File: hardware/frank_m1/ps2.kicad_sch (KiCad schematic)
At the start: 14 parts, among them J4 MDC-036

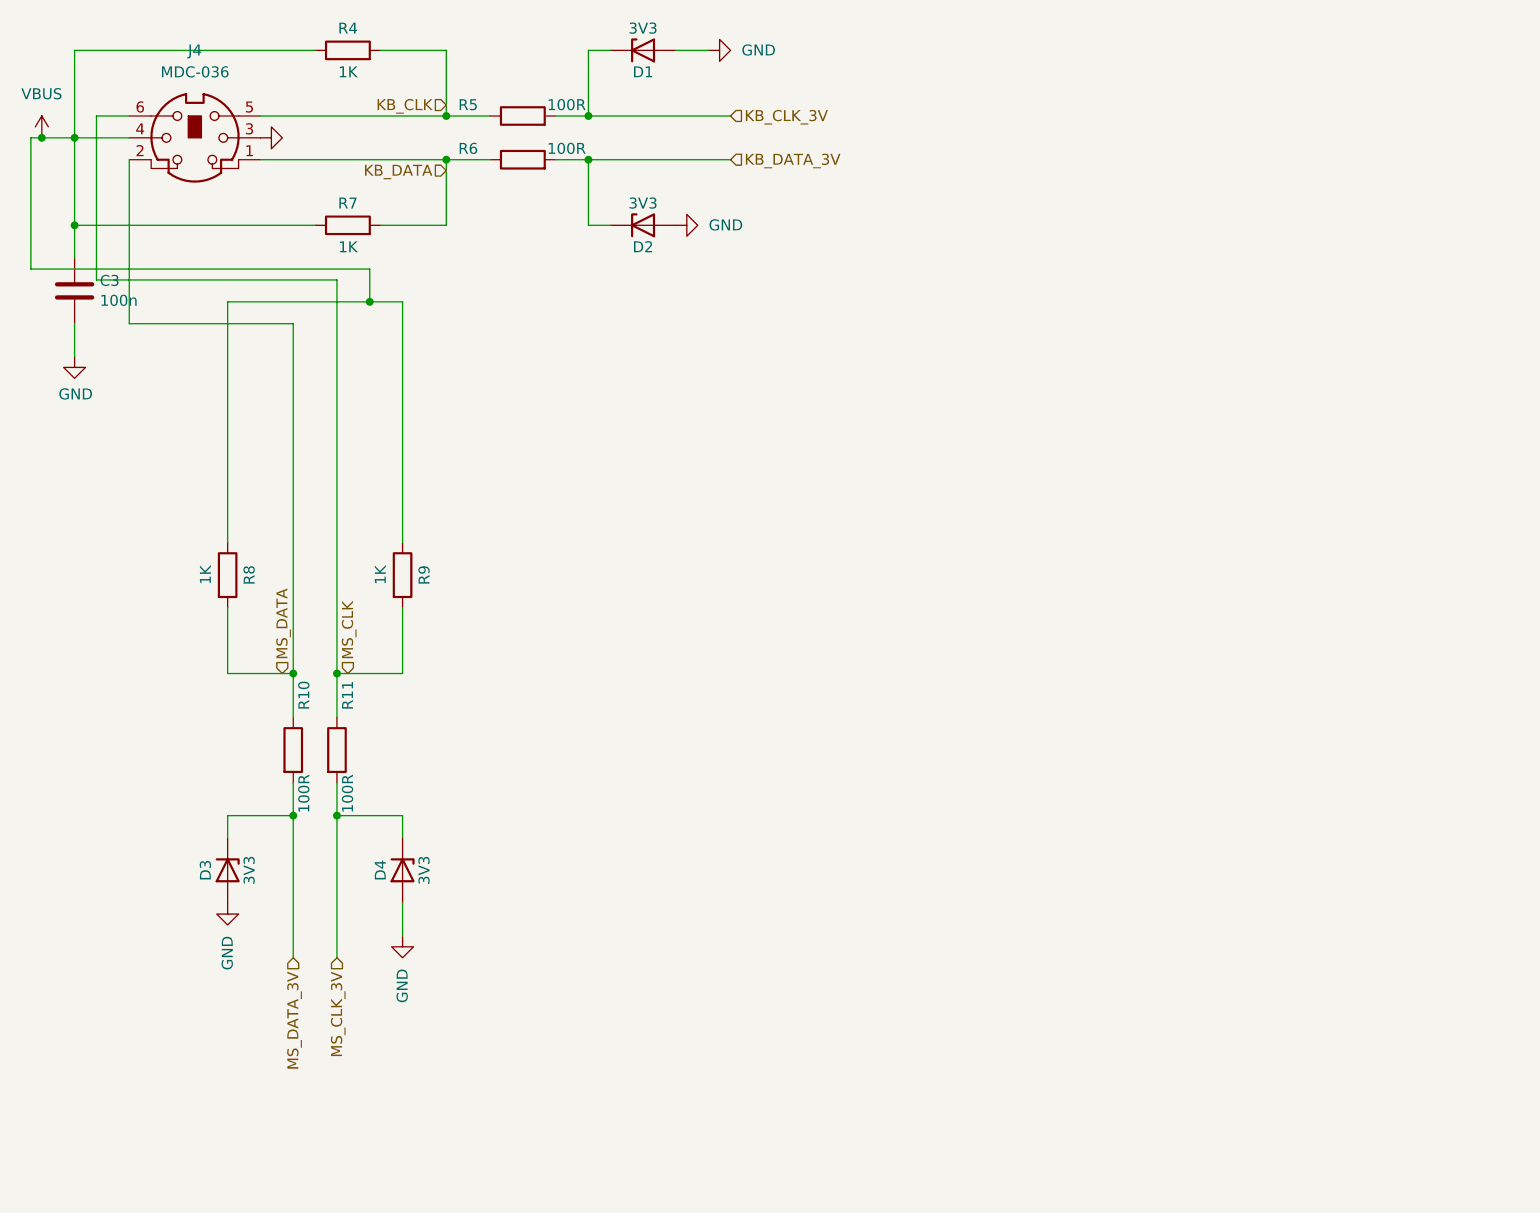
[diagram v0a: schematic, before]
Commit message: Minor updates
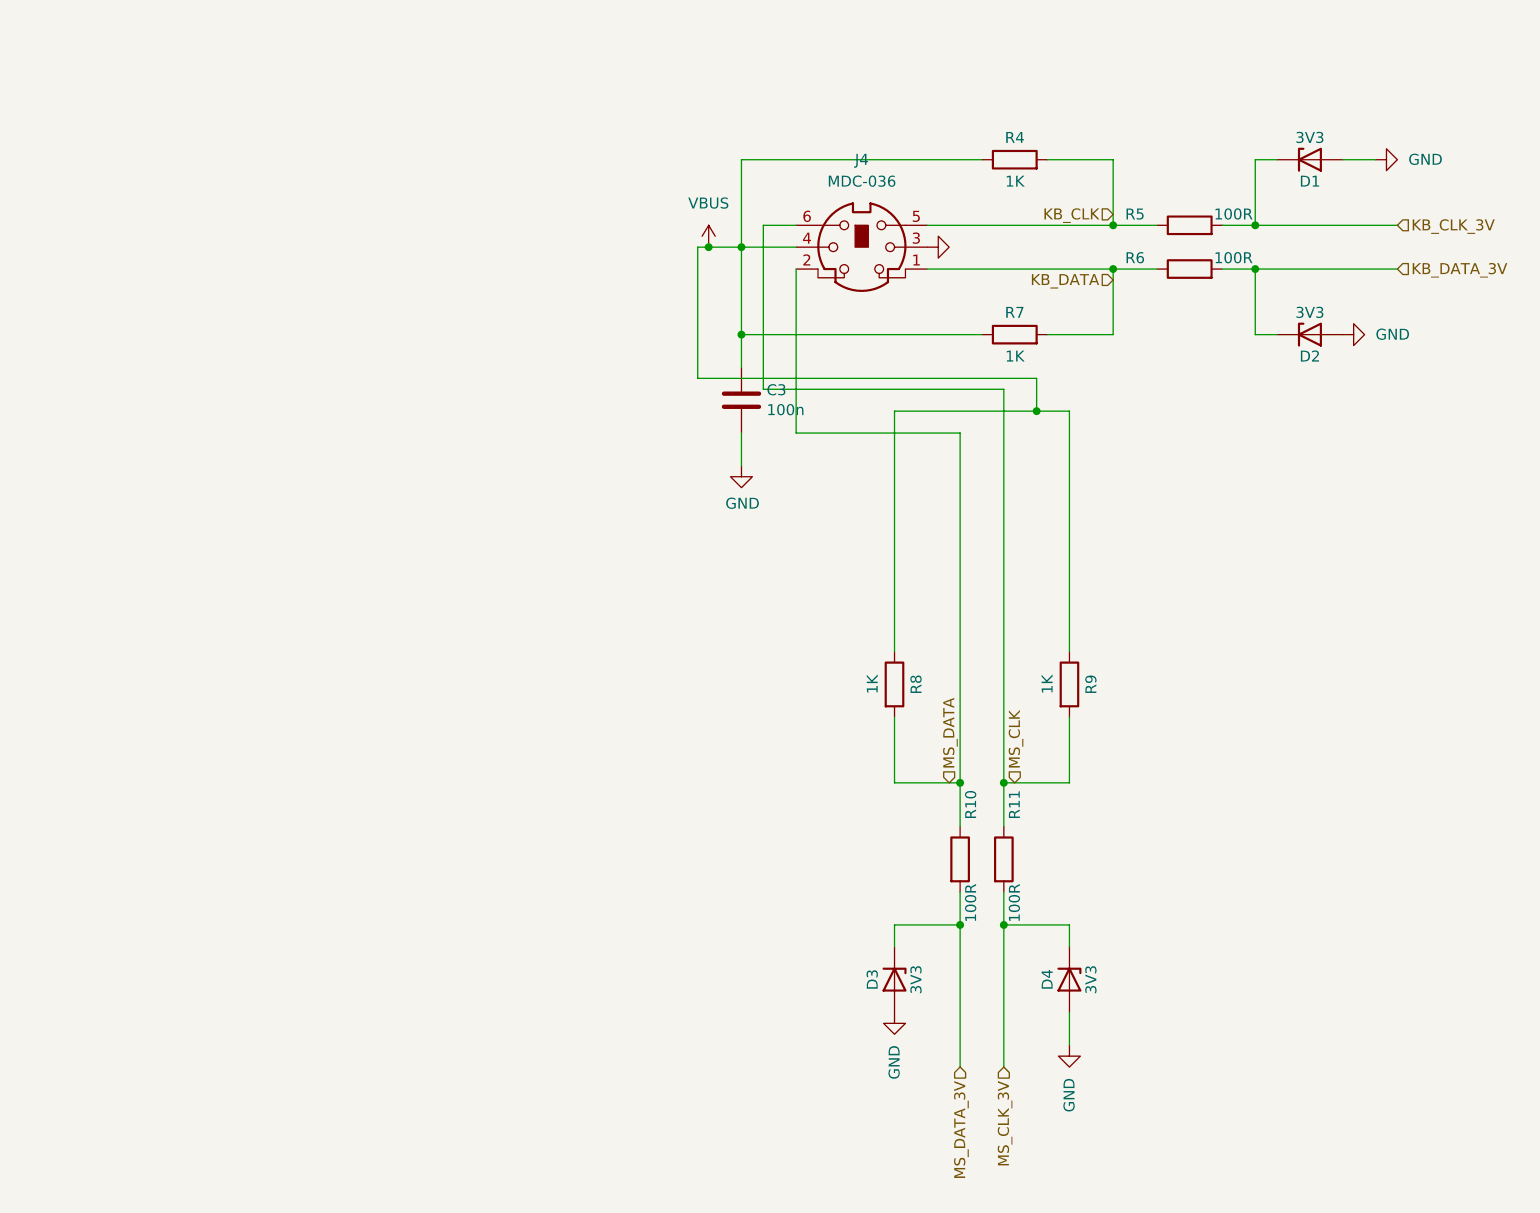
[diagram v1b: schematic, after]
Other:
- moved on the sheet: C3, D1, D2, D3, D4, J4, R10, R11, R4, R5, R6, R7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
